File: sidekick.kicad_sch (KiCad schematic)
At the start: 7 parts, among them SW1 SW_PUSH_6mm_H5mm, SW2 SW_PUSH_6mm_H5mm, U2 module_mpu6050, U3 DM-OLED096-636

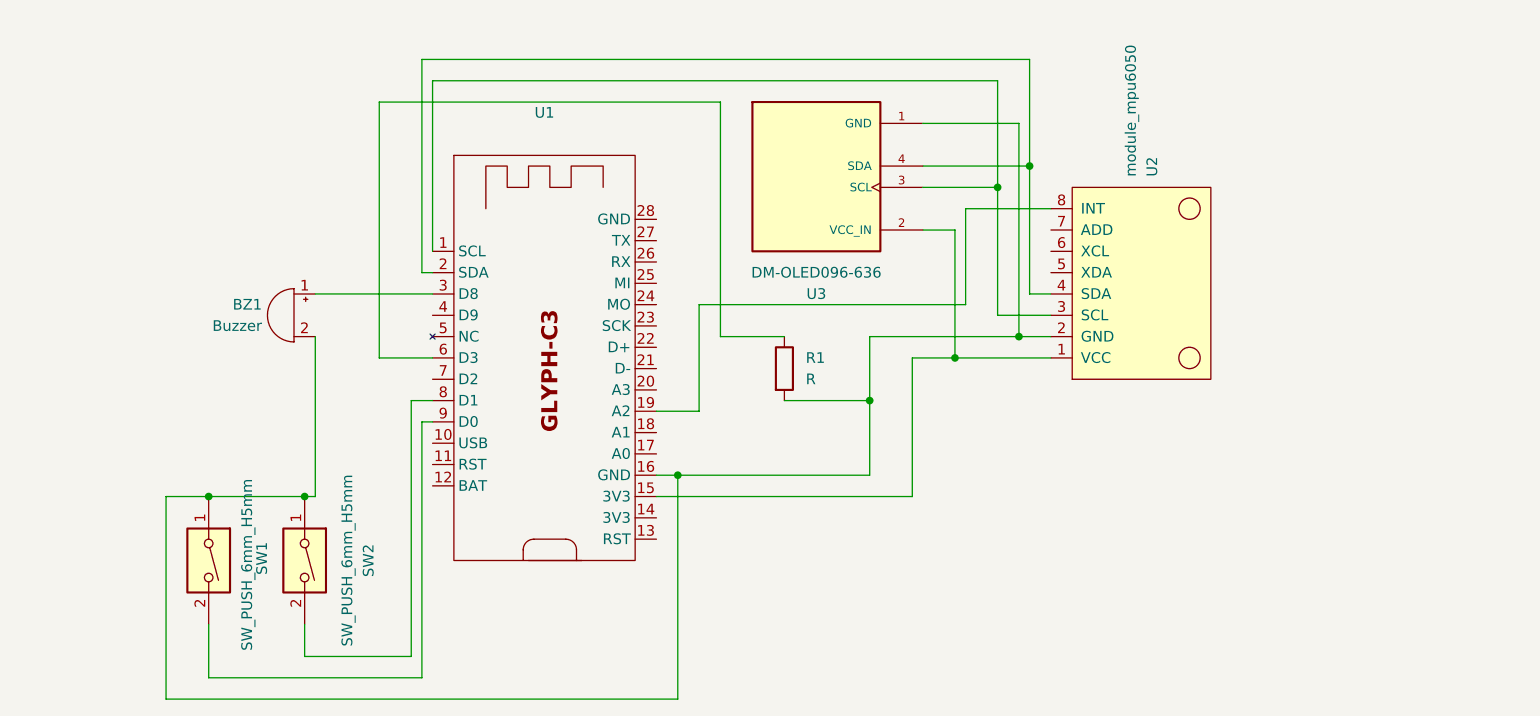
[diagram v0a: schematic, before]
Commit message: Upload v0.3.7 contents
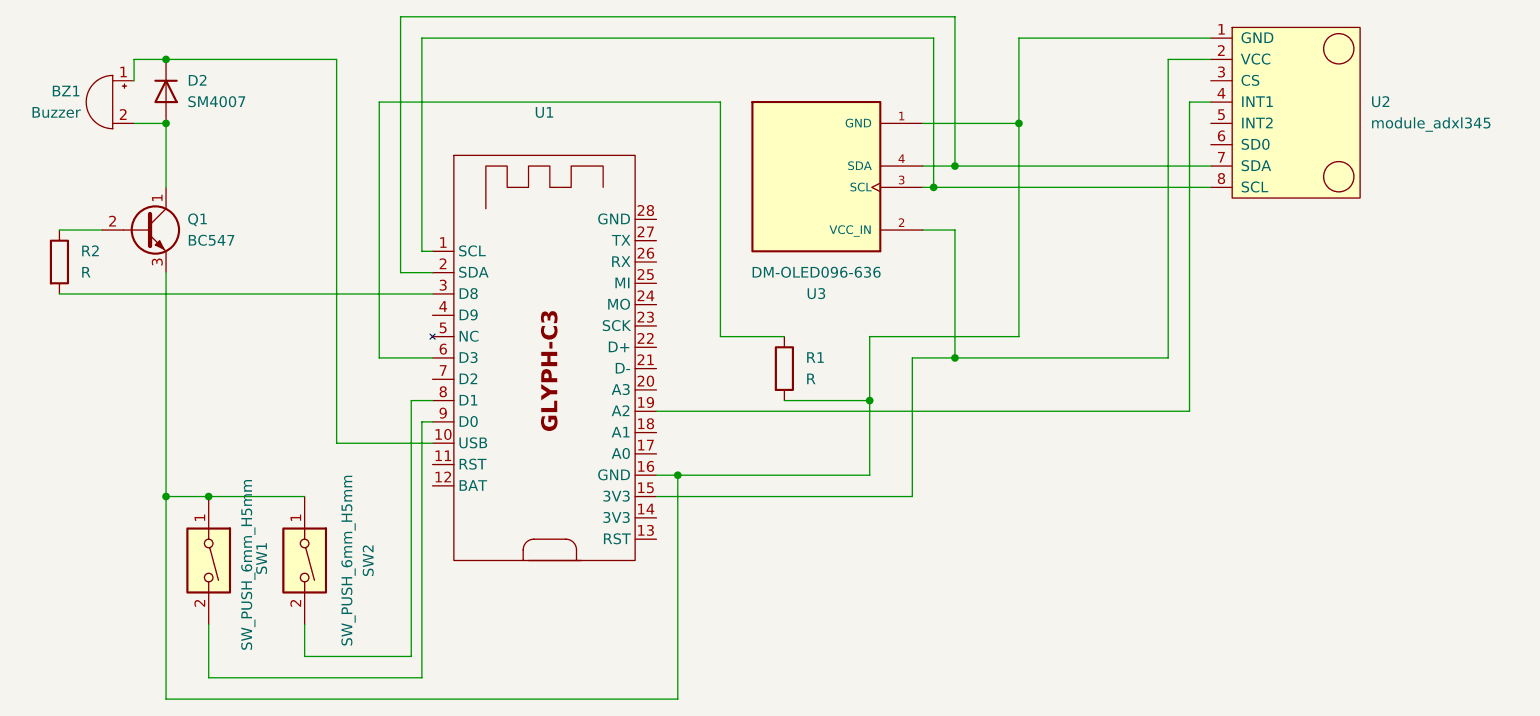
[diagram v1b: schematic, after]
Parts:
- removed U2: module_mpu6050, usini_sensors:module_mpu6050, symbol usini_sensors:module_mpu6050
- added D2: SM4007, Diode_SMD:D_MELF, symbol Diode:SM4007
- added Q1: BC547, Package_TO_SOT_THT:TO-92_Inline, symbol Transistor_BJT:BC547
- added R2: R, Resistor_THT:R_Axial_DIN0204_L3.6mm_D1.6mm_P5.08mm_Horizontal, symbol Device:R
- added U2: module_adxl345, usini_sensors:module_adxl345, symbol usini_sensors:module_adxl345
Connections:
- net at U1.1 (SCL), U3.3 (SCL): now also U2.8 (SCL)
- net at U1.10 (USB): now also BZ1.1 (+), D2.1 (K)
- net at U1.15 (3V3), U3.2 (VCC_IN): now also U2.2 (VCC)
- net at R1.2, SW1.1, SW2.1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: now also Q1.3 (E), U2.1 (GND); no longer BZ1.2 (-)
- net at U1.19 (A2): now also U2.4 (INT1)
- net at U1.2 (SDA), U3.4 (SDA): now also U2.7 (SDA)
- net at U1.3 (D8): now also R2.2; no longer BZ1.1 (+)
- new net: BZ1.2 (-), D2.2 (A), Q1.1 (C)
- new net: Q1.2 (B), R2.1
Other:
- moved on the sheet: BZ1
